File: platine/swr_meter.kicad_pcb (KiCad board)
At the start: 2 copper layers, 16 parts, among them U1 CP0x0xx5425xNTR_Directional_C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, U2 LTC5530, U3 LM1117_SOT223, U4 STM32F030C8Tx

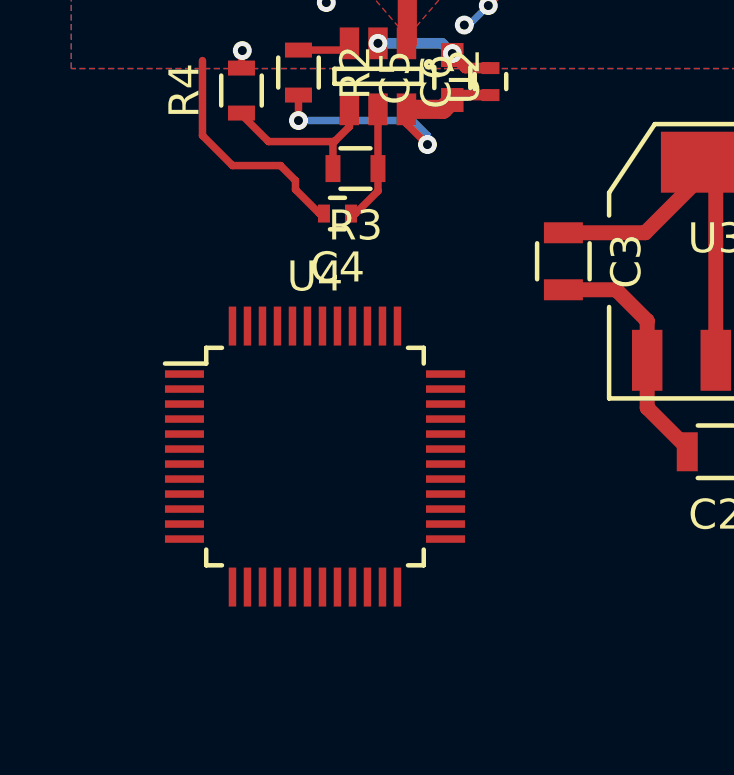
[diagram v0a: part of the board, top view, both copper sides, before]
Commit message: wiring of stm32
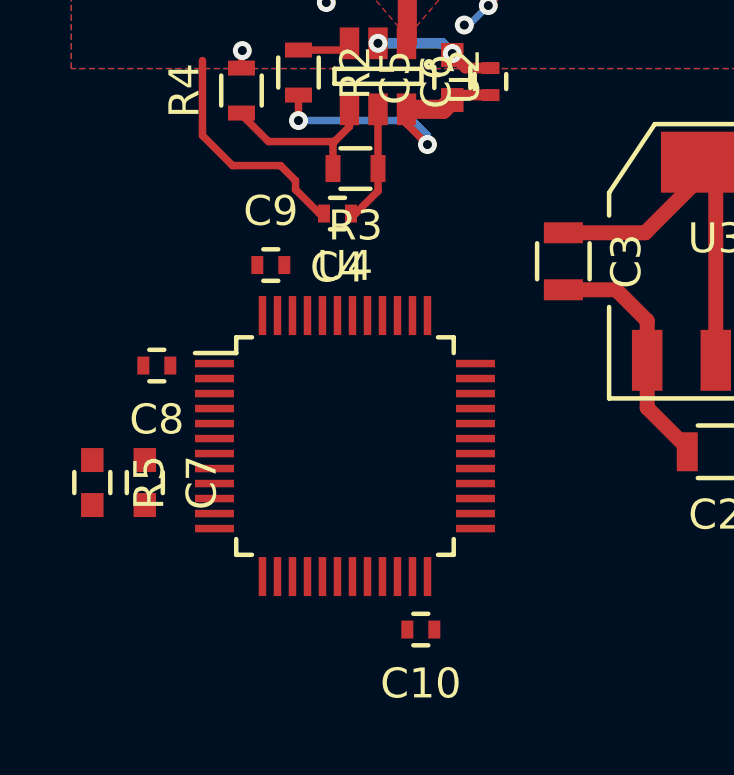
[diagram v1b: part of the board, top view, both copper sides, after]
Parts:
- added C10: 100nF, Resistors_SMD:R_0402, F.Cu at (160.7, 130.2)
- added C7: 1uF, Capacitors_SMD:C_0603, F.Cu at (151.4, 125.3)
- added C8: 100nF, Resistors_SMD:R_0402, F.Cu at (151.8, 121.4)
- added C9: 100nF, Resistors_SMD:R_0402, F.Cu at (155.7, 118.0)
- added R5: 10R, Capacitors_SMD:C_0603, F.Cu at (149.7, 125.3)
- moved U4 1.06 mm to (158.1, 124.1)
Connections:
- net Net-(U4-Pad30) renamed /u1_tx
- net Net-(U4-Pad31) renamed /u1_rx
- net Net-(U4-Pad34) renamed /tms
- net Net-(U4-Pad37) renamed /tck
- net Net-(U4-Pad7) renamed /reset
- C3 pad 1: +5V -> +3V3
- C5 pad 1: +5V -> +3V3
- C6 pad 1: +5V -> +3V3
- R2 pad 2: +5V -> +3V3
- U2 pad 6: +5V -> +3V3
- U3 pad 2: +5V -> +3V3
- U3 pad 4: +5V -> +3V3
- U4 pad 1: Net-(U4-Pad1) -> +3V3
- U4 pad 11: Net-(U4-Pad11) -> Net-(C4-Pad1)
- U4 pad 23: Net-(U4-Pad23) -> GND
- U4 pad 24: Net-(U4-Pad24) -> +3V3
- U4 pad 44: Net-(U4-Pad44) -> GND
- U4 pad 47: Net-(U4-Pad47) -> GND
- U4 pad 48: Net-(U4-Pad48) -> +3V3
- U4 pad 8: Net-(U4-Pad8) -> GND
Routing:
- net +5V: track 22.8 -> 0.00 mm, vias 2 -> 0
- net +3V3: track 0.00 -> 22.8 mm, vias 0 -> 2
